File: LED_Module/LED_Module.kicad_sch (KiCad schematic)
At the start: 55 parts, among them J1 Conn_02x05_Odd_Even, J2 Conn_01x03_Male, J3 ESP8266 Header, J4 Barrel_Jack, SW1 SW_Push, SW2 SW_Push, U1 LD1117S33TR_SOT223, U2 STM32F091RCTx, U3 TPS62A02DRL, U4 24AA32AF EEPROM

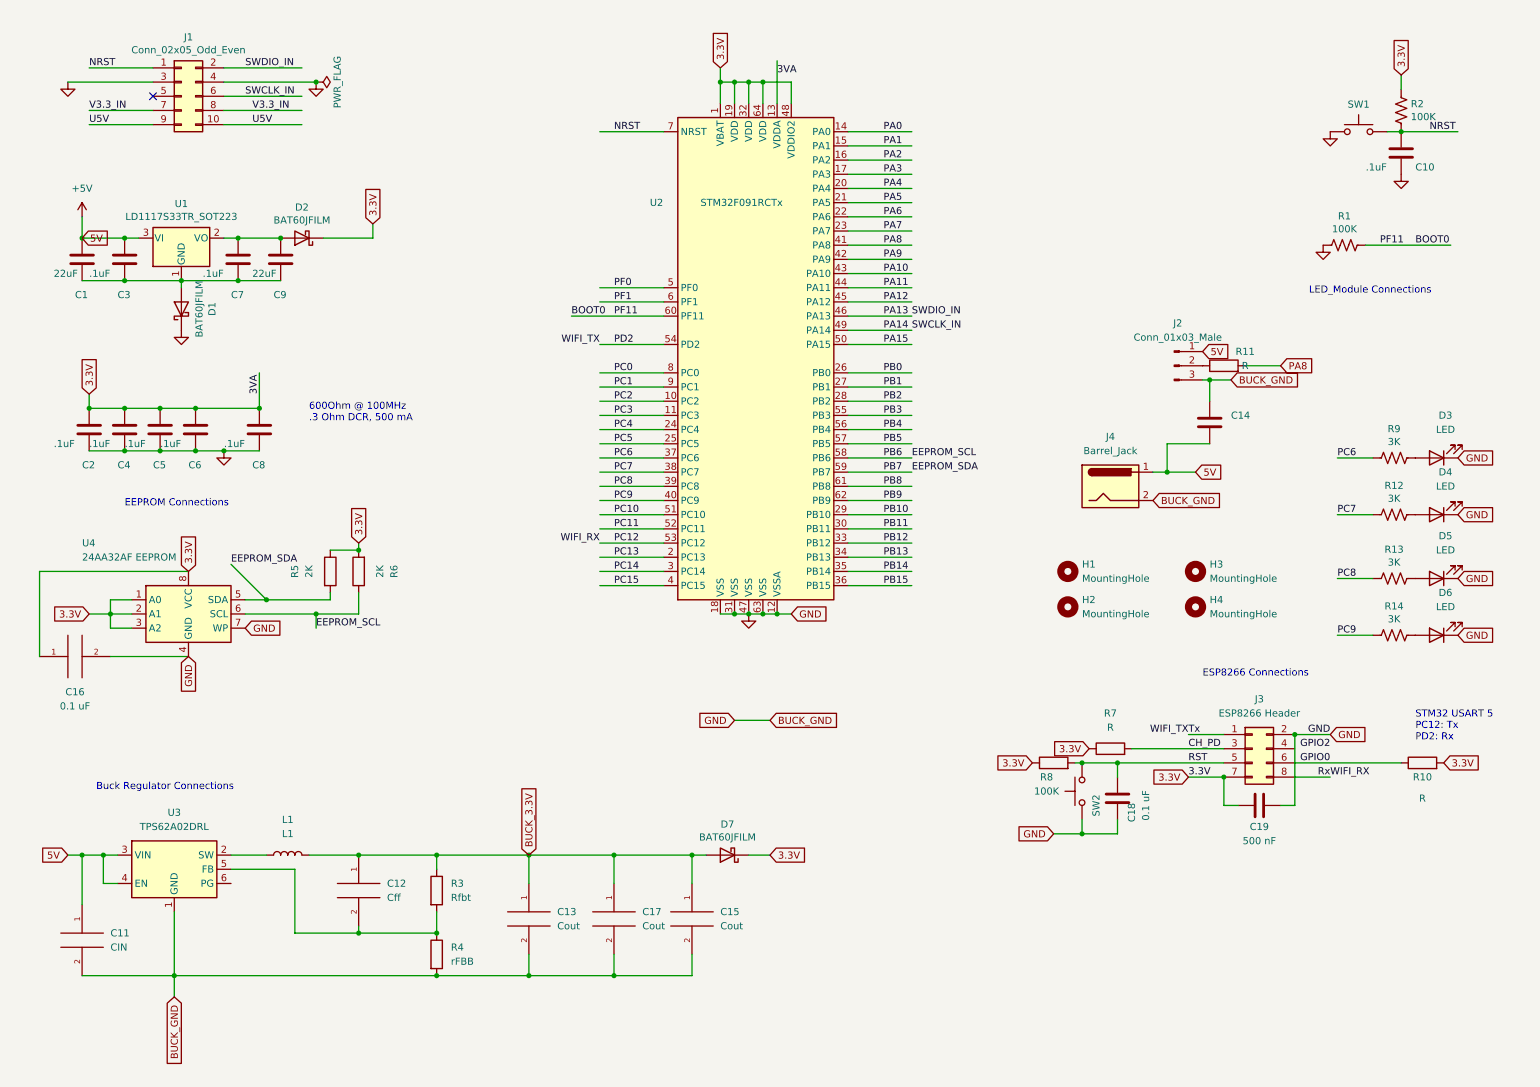
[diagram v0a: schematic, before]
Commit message: PCB design updated for week 8 design review
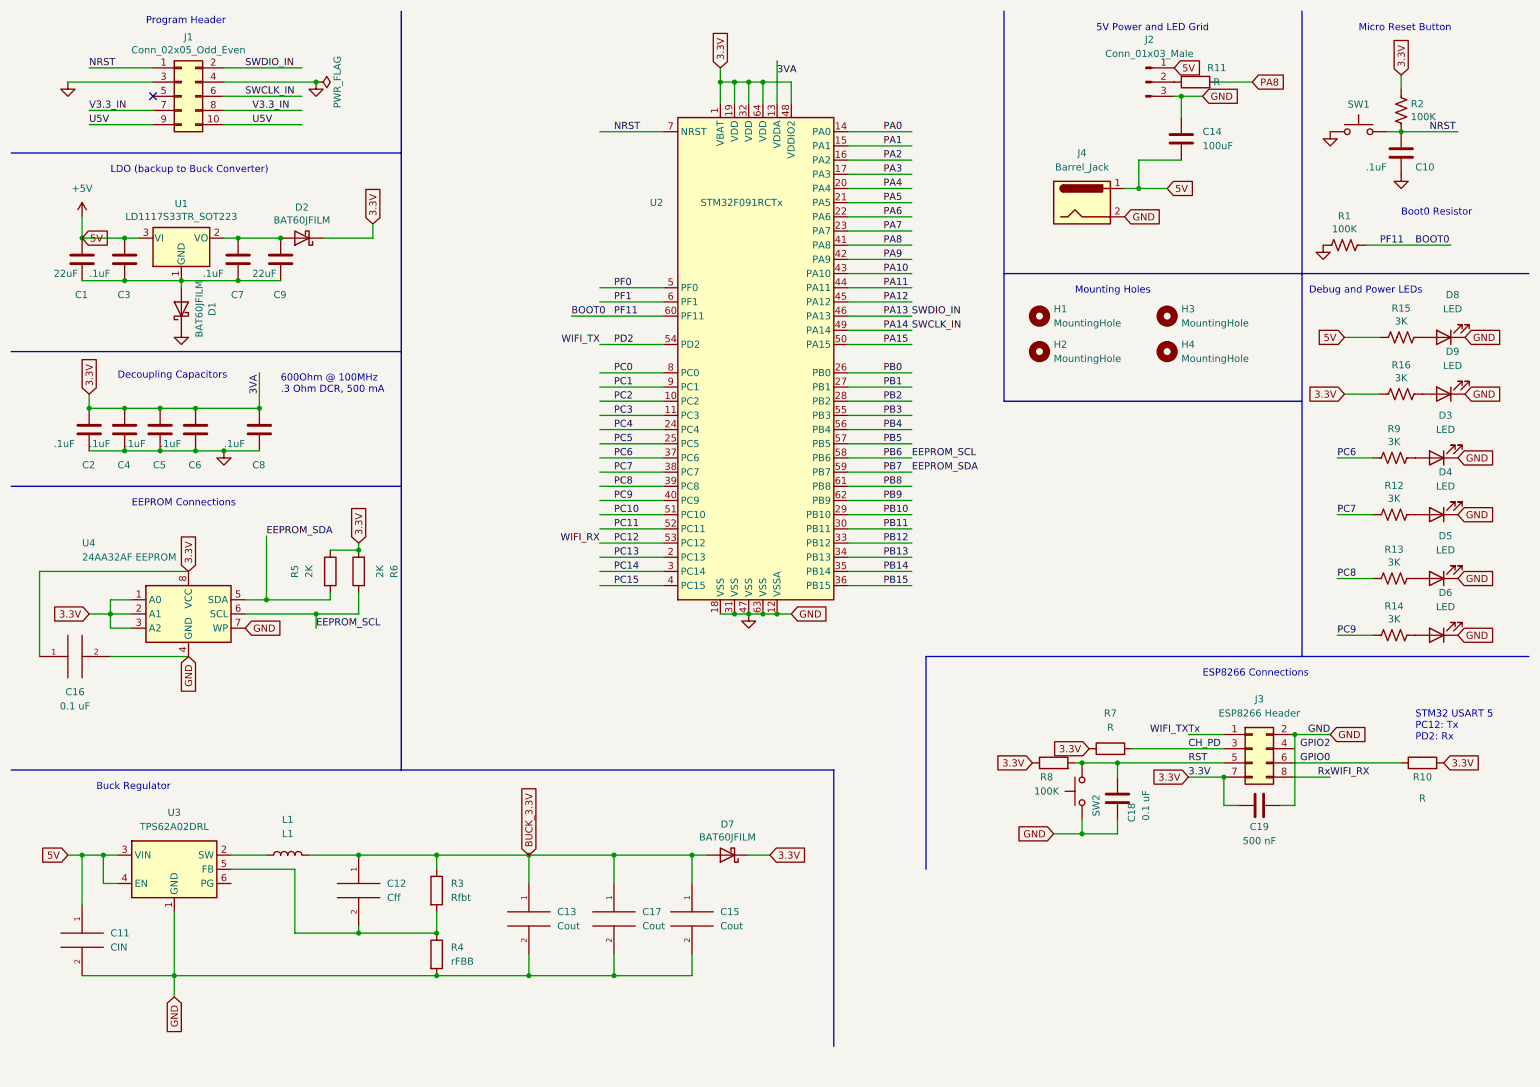
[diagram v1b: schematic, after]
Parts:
- added D8, D9: LED, LED_SMD:LED_0805_2012Metric_Pad1.15x1.40mm_HandSolder, symbol Device:LED
- added R15, R16: 3K, Resistor_SMD:R_0805_2012Metric_Pad1.20x1.40mm_HandSolder, symbol Device:R_US
- C11, C13, C15, C17: footprint Capacitor_SMD:C_0805_2012Metric_Pad1.18x1.45mm_HandSolder -> (none)
- C12: footprint Capacitor_SMD:C_0402_1005Metric_Pad0.74x0.62mm_HandSolder -> (none)
- C14: value (none) -> 100uF; footprint (none) -> Capacitor_THT:C_Rect_L7.0mm_W2.0mm_P5.00mm
- L1: footprint Inductor_SMD:L_0603_1608Metric_Pad1.05x0.95mm_HandSolder -> (none)
- R3, R4: footprint Resistor_SMD:R_0805_2012Metric_Pad1.20x1.40mm_HandSolder -> (none)
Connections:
- net +5V: now also R15.2
- net 3.3V: now also R16.2
- net GND: now also D8.1 (K), D9.1 (K)
- new net: D9.2 (A), R16.1
- new net: D8.2 (A), R15.1
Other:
- note added: "5V Power and LED Grid"
- note added: "Boot0 Resistor"
- note added: "Buck Regulator"
- note added: "Debug and Power LEDs"
- note added: "Decoupling Capacitors"
- note added: "LDO (backup to Buck Converter)"
- note added: "Micro Reset Button"
- note added: "Mounting Holes"
- note added: "Program Header"
- note removed: "Buck Regulator Connections"
- note removed: "LED_Module Connections"
- moved on the sheet: C14, H1, H2, H3, H4, J2, J4, R11
